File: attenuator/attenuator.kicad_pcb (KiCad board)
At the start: 2 copper layers, 80 x 33.1 mm, 65 parts, among them J1 Conn_Coaxial, J2 Conn_Coaxial, J3 Conn_02x07_Odd_Even, U1 4259-63, U10 4259-63, U2 4259-63, U3 4259-63, U4 4259-63, U5 4259-63, U6 4259-63, U7 4259-63, U8 4259-63, U9 4259-63

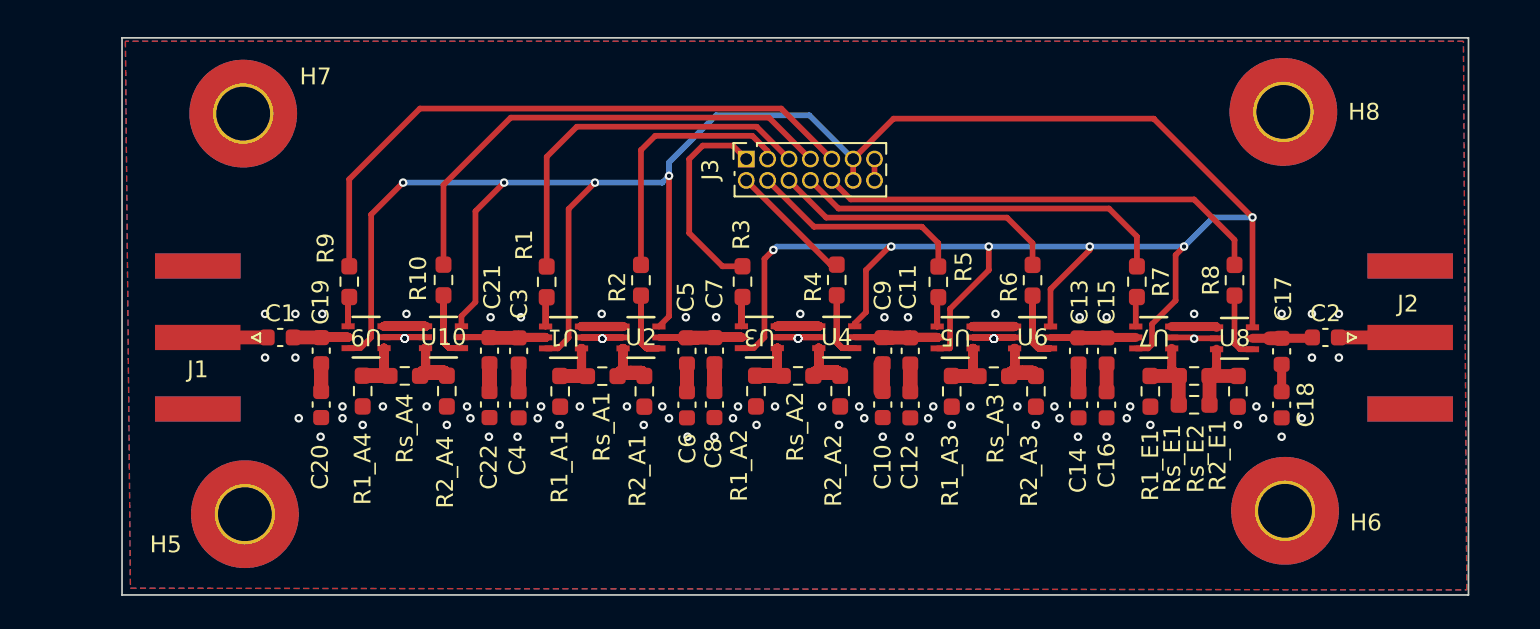
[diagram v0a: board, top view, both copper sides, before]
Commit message: finish simulation and kicad
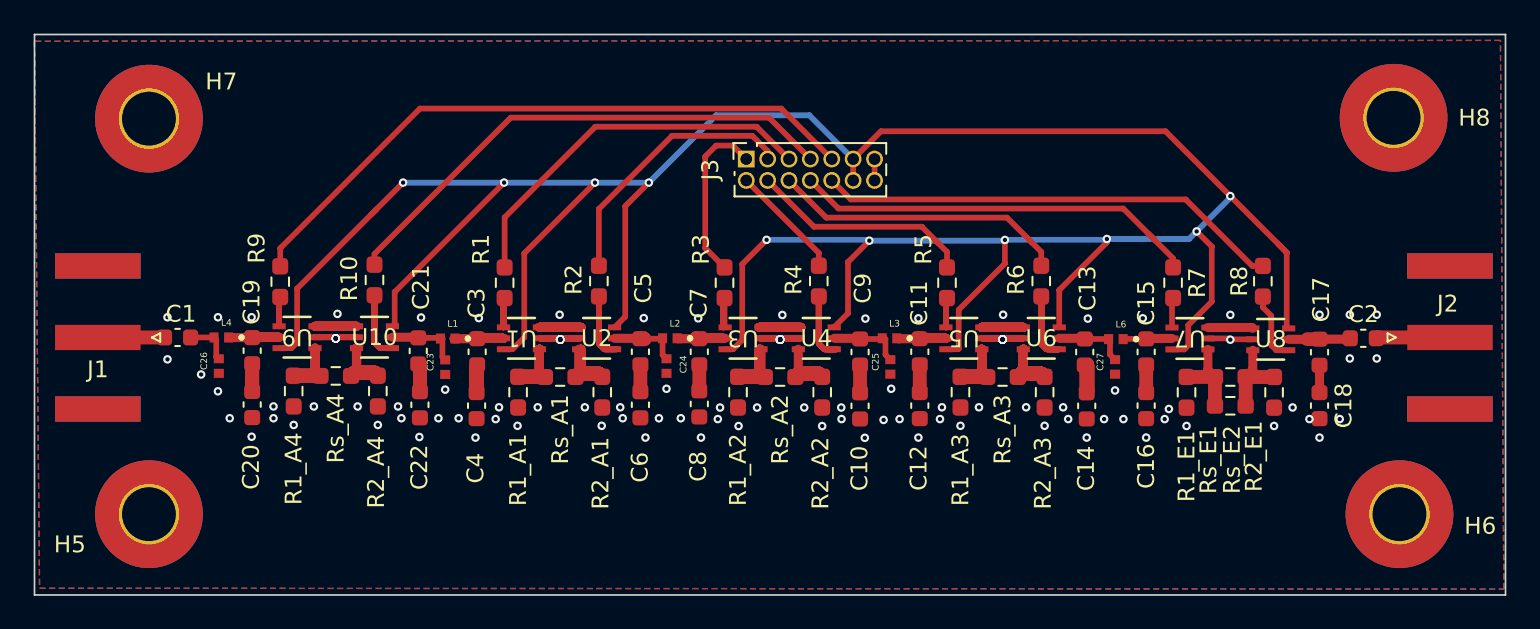
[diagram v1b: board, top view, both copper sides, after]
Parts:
- added C23: GCQ1555C1HR85WB01D, attenuator:CAPC1005X55N, F.Cu at (50.1, 45.6)
- added C24: GCQ1555C1HR85WB01D, attenuator:CAPC1005X55N, F.Cu at (63.2, 45.5)
- added C25: GCQ1555C1HR85WB01D, attenuator:CAPC1005X55N, F.Cu at (76.5, 45.5)
- added C26: GCQ1555C1HR85WB01D, attenuator:CAPC1005X55N, F.Cu at (36.6, 45.5)
- added C27: GCQ1555C1HR85WB01D, attenuator:CAPC1005X55N, F.Cu at (89.9, 45.5)
- added L1: LQG15HN2N0S02D, attenuator:INDC1005X55N, F.Cu at (50.2, 43.9)
- added L2: LQG15HN2N0S02D, attenuator:INDC1005X55N, F.Cu at (63.5, 43.9)
- added L3: LQG15HN2N0S02D, attenuator:INDC1005X55N, F.Cu at (76.5, 43.9)
- added L4: LQG15HN2N0S02D, attenuator:INDC1005X55N, F.Cu at (36.8, 43.8)
- added L6: LQG15HN2N0S02D, attenuator:INDC1005X55N, F.Cu at (90.0, 43.9)
- moved H6 6.80 mm to (106.8, 54.3)
- moved H8 6.56 mm to (106.5, 30.8)
- moved C1 6.10 mm to (34.2, 43.8)
- moved J1 5.94 mm to (29.5, 43.8)
- moved H5 5.70 mm to (32.5, 54.3)
- moved H7 5.61 mm to (32.5, 30.8)
- moved C21 4.23 mm to (48.5, 44.6)
- moved C22 4.13 mm to (48.6, 47.8)
- moved R10 4.10 mm to (45.9, 40.4)
- moved R1_A4 4.10 mm to (41.1, 47.0)
- moved R2_A4 4.10 mm to (46.1, 47.0)
- moved R9 4.10 mm to (40.3, 40.5)
- moved Rs_A4 4.10 mm to (43.6, 46.1)
- moved U10 4.10 mm to (45.9, 43.8)
- moved U9 4.10 mm to (41.3, 43.8)
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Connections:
- C11 pad 1: /attenuator_block2/RFC_OUT -> Net-(U5-RFC)
- C15 pad 1: /attenuator_block3/RFC_OUT -> Net-(U7-RFC)
- C19 pad 1: /attenuator_block/RFC_IN -> Net-(U9-RFC)
- C3 pad 1: /attenuator_block/RFC_OUT -> Net-(U1-RFC)
- C7 pad 1: /attenuator_block1/RFC_OUT -> Net-(U3-RFC)
- U1 pad 5: /attenuator_block/RFC_OUT -> Net-(U1-RFC)
- U3 pad 5: /attenuator_block1/RFC_OUT -> Net-(U3-RFC)
- U5 pad 5: /attenuator_block2/RFC_OUT -> Net-(U5-RFC)
- U7 pad 5: /attenuator_block3/RFC_OUT -> Net-(U7-RFC)
- U9 pad 5: /attenuator_block/RFC_IN -> Net-(U9-RFC)
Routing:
- net GND: track 52.0 -> 82.0 mm, vias 93 -> 118
- net Net-(U3-RFC): track 0.00 -> 17.6 mm
- net Net-(U5-RFC): track 0.00 -> 17.5 mm
- net Net-(U6-CTRL): track 24.1 -> 40.1 mm
- net Net-(U2-CTRL): track 12.0 -> 27.9 mm
- net Net-(U4-CTRL): track 24.1 -> 39.9 mm
- net Net-(U1-RF1): track 11.0 -> 25.6 mm
- net Net-(U5-RF1): track 22.0 -> 36.6 mm
- net Net-(U3-RF1): track 22.0 -> 36.6 mm
- net Net-(U6-RF2): track 21.2 -> 35.3 mm
- net Net-(U2-RF2): track 10.6 -> 24.7 mm
- net Net-(U1-RFC): track 0.00 -> 12.7 mm
- net Net-(U5-RF2): track 14.8 -> 24.7 mm
- net Net-(U1-RF2): track 7.40 -> 17.1 mm
- net Net-(U3-RF2): track 14.8 -> 24.3 mm
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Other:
- board size 80 x 33.1 mm -> 87.4 x 33.3 mm
